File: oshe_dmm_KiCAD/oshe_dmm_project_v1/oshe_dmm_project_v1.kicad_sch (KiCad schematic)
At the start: 65 parts, among them J1 FTDI Basic, J2 USB_C_Receptacle_PowerOnly_6P, J3 ON/OFF, J4 Conn_01x16, SW1 SW_Push, SW2 SW_Rotary_1x4_MP, U1 ATmega328P-A, U2 INA219BxD, U3 BQ24075RGT, U4 LM317_SOT-223, U5 ADS1115IDGS, Y1 16MHz

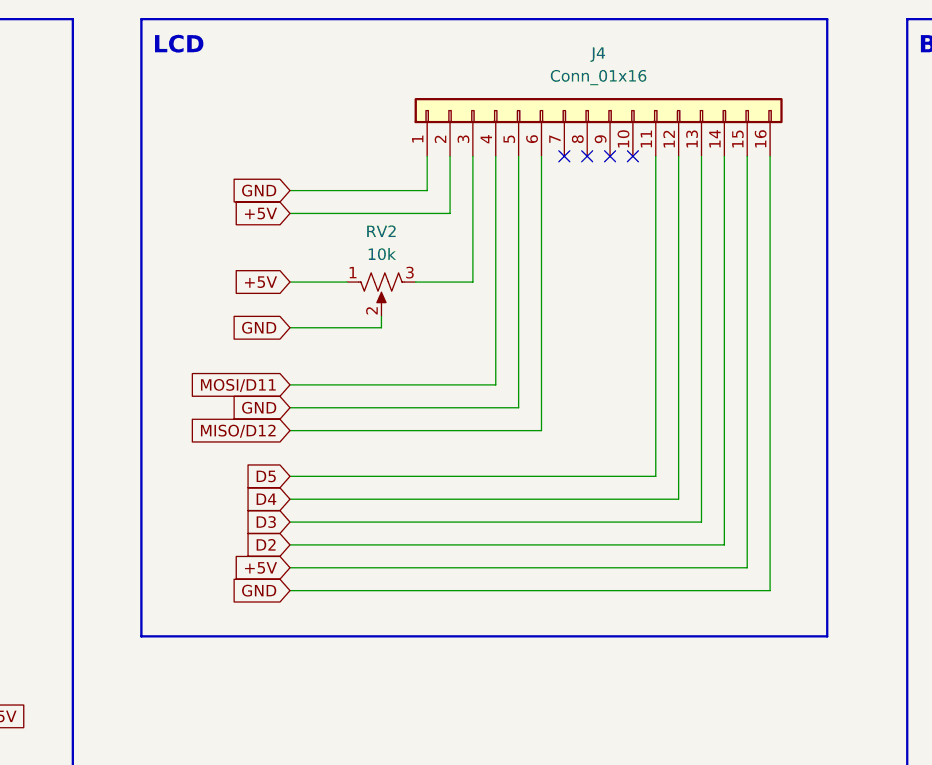
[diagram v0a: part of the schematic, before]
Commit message: made some more changes!
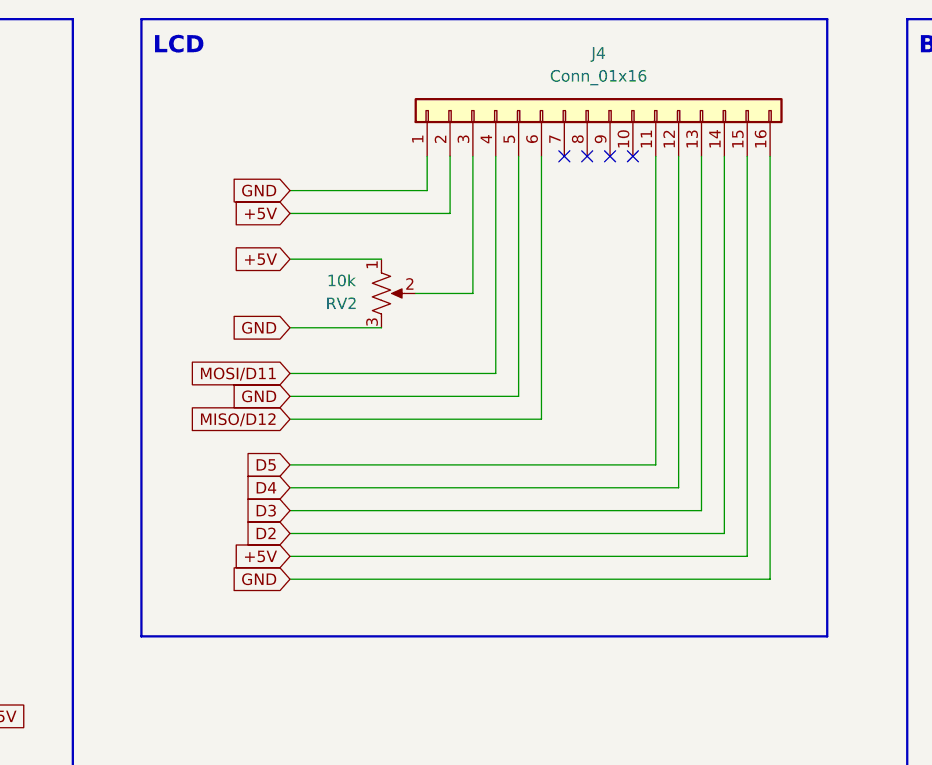
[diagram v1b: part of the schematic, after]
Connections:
- net GND: now also RV2.3; no longer RV2.2
- net at J4.3 (Pin_3): now also RV2.2; no longer RV2.3
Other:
- moved on the sheet: RV2
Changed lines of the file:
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@@
 	(wire
 		(pts
+			(xy 166.37 45.72) (xy 172.72 45.72)
+		)
+		(stroke
+			(width 0)
+			(type default)
+		)
+	)
+	(wire
+		(pts
 			(xy 332.74 41.91) (xy 345.44 41.91)
 		)
@@
 	(wire
 		(pts
-			(xy 152.4 73.66) (xy 200.66 73.66)
+			(xy 152.4 72.39) (xy 200.66 72.39)
+		)
+		(stroke
+			(width 0)
+			(type default)
+		)
+	)
+	(wire
+		(pts
+			(xy 152.4 49.53) (xy 162.56 49.53)
 		)
 		(stroke
@@
 	(wire
 		(pts
-			(xy 205.74 78.74) (xy 205.74 30.48)
+			(xy 205.74 77.47) (xy 205.74 30.48)
 		)
 		(stroke
@@
 	(wire
 		(pts
-			(xy 152.4 44.45) (xy 158.75 44.45)
-		)
-		(stroke
-			(width 0)
-			(type default)
-		)
-	)
-	(wire
-		(pts
 			(xy 243.84 111.76) (xy 254 111.76)
 		)
@@
 	(wire
 		(pts
-			(xy 193.04 66.04) (xy 193.04 30.48)
+			(xy 193.04 64.77) (xy 193.04 30.48)
 		)
 		(stroke
@@
 	(wire
 		(pts
-			(xy 152.4 60.96) (xy 180.34 60.96)
+			(xy 152.4 59.69) (xy 180.34 59.69)
 		)
 		(stroke
@@
 	(wire
 		(pts
-			(xy 175.26 55.88) (xy 175.26 30.48)
+			(xy 175.26 54.61) (xy 175.26 30.48)
 		)
 		(stroke
@@
 	(wire
 		(pts
-			(xy 152.4 71.12) (xy 198.12 71.12)
+			(xy 152.4 69.85) (xy 198.12 69.85)
 		)
 		(stroke
@@
 	(wire
 		(pts
-			(xy 152.4 58.42) (xy 177.8 58.42)
+			(xy 152.4 57.15) (xy 177.8 57.15)
 		)
 		(stroke
@@
 	(wire
 		(pts
-			(xy 152.4 49.53) (xy 162.56 49.53)
-		)
-		(stroke
-			(width 0)
-			(type default)
-		)
-	)
-	(wire
-		(pts
 			(xy 233.68 58.42) (xy 233.68 60.96)
 		)
@@
 	(wire
 		(pts
-			(xy 195.58 68.58) (xy 195.58 30.48)
+			(xy 195.58 67.31) (xy 195.58 30.48)
 		)
 		(stroke
@@
 	(wire
 		(pts
-			(xy 180.34 60.96) (xy 180.34 30.48)
+			(xy 180.34 59.69) (xy 180.34 30.48)
 		)
 		(stroke
@@
 	(wire
 		(pts
-			(xy 152.4 66.04) (xy 193.04 66.04)
+			(xy 152.4 64.77) (xy 193.04 64.77)
 		)
 		(stroke
@@
 	(wire
 		(pts
+			(xy 172.72 45.72) (xy 172.72 30.48)
+		)
+		(stroke
+			(width 0)
+			(type default)
+		)
+	)
+	(wire
+		(pts
 			(xy 66.04 142.24) (xy 66.04 146.05)
 		)
@@
 	(wire
 		(pts
-			(xy 152.4 55.88) (xy 175.26 55.88)
+			(xy 152.4 54.61) (xy 175.26 54.61)
 		)
 		(stroke
@@
 	(wire
 		(pts
+			(xy 152.4 41.91) (xy 162.56 41.91)
+		)
+		(stroke
+			(width 0)
+			(type default)
+		)
+	)
+	(wire
+		(pts
 			(xy 76.2 161.29) (xy 80.01 161.29)
 		)
@@
 	(wire
 		(pts
-			(xy 152.4 78.74) (xy 205.74 78.74)
+			(xy 152.4 77.47) (xy 205.74 77.47)
 		)
 		(stroke
@@
 	(wire
 		(pts
-			(xy 172.72 44.45) (xy 172.72 30.48)
-		)
-		(stroke
-			(width 0)
-			(type default)
-		)
-	)
-	(wire
-		(pts
 			(xy 261.62 33.02) (xy 285.75 33.02)
 		)
@@
 	(wire
 		(pts
-			(xy 203.2 76.2) (xy 152.4 76.2)
+			(xy 203.2 74.93) (xy 152.4 74.93)
 		)
 		(stroke
@@
 	(wire
 		(pts
-			(xy 152.4 68.58) (xy 195.58 68.58)
+			(xy 152.4 67.31) (xy 195.58 67.31)
 		)
 		(stroke
@@
 	(wire
 		(pts
-			(xy 200.66 73.66) (xy 200.66 30.48)
+			(xy 200.66 72.39) (xy 200.66 30.48)
 		)
 		(stroke
@@
 	(wire
 		(pts
-			(xy 166.37 44.45) (xy 172.72 44.45)
-		)
-		(stroke
-			(width 0)
-			(type default)
-		)
-	)
-	(wire
-		(pts
 			(xy 332.74 49.53) (xy 336.55 49.53)
 		)
@@
 	(wire
 		(pts
-			(xy 177.8 58.42) (xy 177.8 30.48)
+			(xy 177.8 57.15) (xy 177.8 30.48)
 		)
 		(stroke
@@
 	(wire
 		(pts
-			(xy 198.12 71.12) (xy 198.12 30.48)
+			(xy 198.12 69.85) (xy 198.12 30.48)
 		)
 		(stroke
@@
 	(wire
 		(pts
-			(xy 203.2 30.48) (xy 203.2 76.2)
+			(xy 203.2 30.48) (xy 203.2 74.93)
 		)
 		(stroke
@@
 	(wire
 		(pts
-			(xy 162.56 49.53) (xy 162.56 48.26)
-		)
-		(stroke
-			(width 0)
-			(type default)
-		)
-	)
-	(wire
-		(pts
 			(xy 228.6 157.48) (xy 198.12 157.48)
 		)
@@
 	(global_label "GND"
 		(shape input)
-		(at 152.4 78.74 180)
+		(at 152.4 77.47 180)
 		(fields_autoplaced yes)
 		(effects
@@
 		)
 		(property "Intersheetrefs" "${INTERSHEET_REFS}"
-			(at 145.5443 78.74 0)
+			(at 145.5443 77.47 0)
 			(effects
 				(font
@@
 	(global_label "D5"
 		(shape input)
-		(at 152.4 66.04 180)
+		(at 152.4 64.77 180)
 		(fields_autoplaced yes)
 		(effects
@@
 		)
 		(property "Intersheetrefs" "${INTERSHEET_REFS}"
-			(at 146.9353 66.04 0)
+			(at 146.9353 64.77 0)
 			(effects
 				(font
@@
 	(global_label "GND"
 		(shape input)
-		(at 152.4 58.42 180)
+		(at 152.4 57.15 180)
 		(fields_autoplaced yes)
 		(effects
@@
 		)
 		(property "Intersheetrefs" "${INTERSHEET_REFS}"
-			(at 145.5443 58.42 0)
+			(at 145.5443 57.15 0)
 			(effects
 				(font
@@
 	(global_label "+5V"
 		(shape input)
-		(at 152.4 76.2 180)
+		(at 152.4 74.93 180)
 		(fields_autoplaced yes)
 		(effects
@@
 		)
 		(property "Intersheetrefs" "${INTERSHEET_REFS}"
-			(at 145.5443 76.2 0)
+			(at 145.5443 74.93 0)
 			(effects
 				(font
@@
 	(global_label "MISO{slash}D12"
 		(shape input)
-		(at 152.4 60.96 180)
+		(at 152.4 59.69 180)
 		(fields_autoplaced yes)
 		(effects
@@
 		)
 		(property "Intersheetrefs" "${INTERSHEET_REFS}"
-			(at 139.7991 60.96 0)
+			(at 139.7991 59.69 0)
 			(effects
 				(font
@@
 	(global_label "D4"
 		(shape input)
-		(at 152.4 68.58 180)
+		(at 152.4 67.31 180)
 		(fields_autoplaced yes)
 		(effects
@@
 		)
 		(property "Intersheetrefs" "${INTERSHEET_REFS}"
-			(at 146.9353 68.58 0)
+			(at 146.9353 67.31 0)
 			(effects
 				(font
@@
 	(global_label "D3"
 		(shape input)
-		(at 152.4 71.12 180)
+		(at 152.4 69.85 180)
 		(fields_autoplaced yes)
 		(effects
@@
 		)
 		(property "Intersheetrefs" "${INTERSHEET_REFS}"
-			(at 146.9353 71.12 0)
+			(at 146.9353 69.85 0)
 			(effects
 				(font
@@
 	(global_label "D2"
 		(shape input)
-		(at 152.4 73.66 180)
+		(at 152.4 72.39 180)
 		(fields_autoplaced yes)
 		(effects
@@
 		)
 		(property "Intersheetrefs" "${INTERSHEET_REFS}"
-			(at 146.9353 73.66 0)
+			(at 146.9353 72.39 0)
 			(effects
 				(font
@@
 	(global_label "+5V"
 		(shape input)
-		(at 152.4 44.45 180)
+		(at 152.4 41.91 180)
 		(fields_autoplaced yes)
 		(effects
@@
 		)
 		(property "Intersheetrefs" "${INTERSHEET_REFS}"
-			(at 145.5443 44.45 0)
+			(at 145.5443 41.91 0)
 			(effects
 				(font
@@
 	(global_label "MOSI{slash}D11"
 		(shape input)
-		(at 152.4 55.88 180)
+		(at 152.4 54.61 180)
 		(fields_autoplaced yes)
 		(effects
@@
 		)
 		(property "Intersheetrefs" "${INTERSHEET_REFS}"
-			(at 139.7991 55.88 0)
+			(at 139.7991 54.61 0)
 			(effects
 				(font
@@
 	(symbol
 		(lib_id "Device:R_Potentiometer_US")
-		(at 162.56 44.45 90)
-		(mirror x)
+		(at 162.56 45.72 0)
 		(unit 1)
 		(exclude_from_sim no)
@@
 		(dnp no)
 		(property "Reference" "RV2"
-			(at 162.56 38.862 90)
+			(at 158.115 46.863 0)
 			(effects
 				(font
@@
 		)
 		(property "Value" "10k"
-			(at 162.56 41.402 90)
+			(at 158.115 44.323 0)
 			(effects
 				(font
@@
 		)
 		(property "Footprint" "Potentiometer_SMD:Potentiometer_ACP_CA6-VSMD_Vertical"
-			(at 162.56 44.45 0)
+			(at 162.56 45.72 0)
 			(effects
 				(font
@@
 		)
 		(property "Datasheet" "~"
-			(at 162.56 44.45 0)
+			(at 162.56 45.72 0)
 			(effects
 				(font
@@
 		)
 		(property "Description" "Potentiometer, US symbol"
-			(at 162.56 44.45 0)
+			(at 162.56 45.72 0)
 			(effects
 				(font
